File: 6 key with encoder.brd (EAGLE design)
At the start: 96.4 x 40.5 mm, 25 parts, among them SW1 KEYSWITCH-PLAIN-MXHS-1U, SW2 KEYSWITCH-PLAIN-MXHS-1U, SW3 KEYSWITCH-PLAIN-MXHS-1U, SW4 KEYSWITCH-PLAIN-MXHS-1U, SW5 KEYSWITCH-PLAIN-MXHS-1U, SW6 KEYSWITCH-PLAIN-MXHS-1U

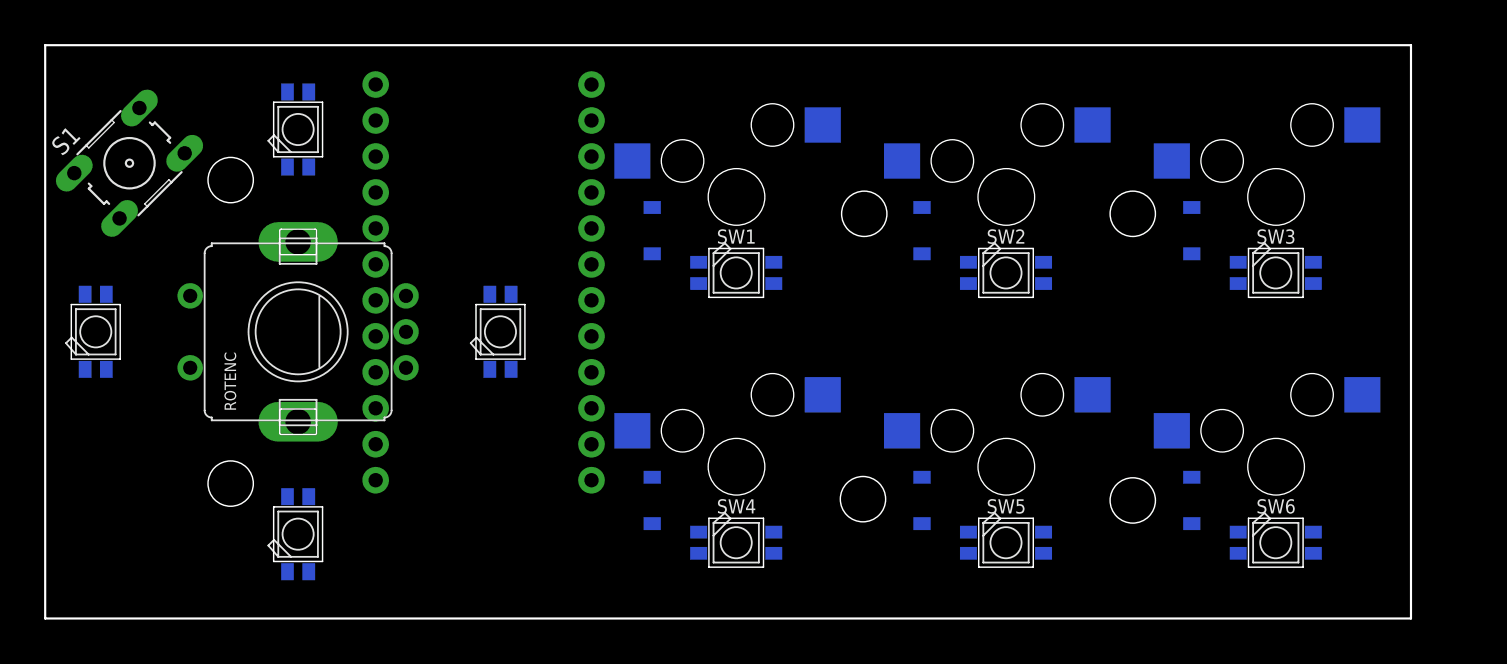
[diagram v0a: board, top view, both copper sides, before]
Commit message: production 12-6-2021
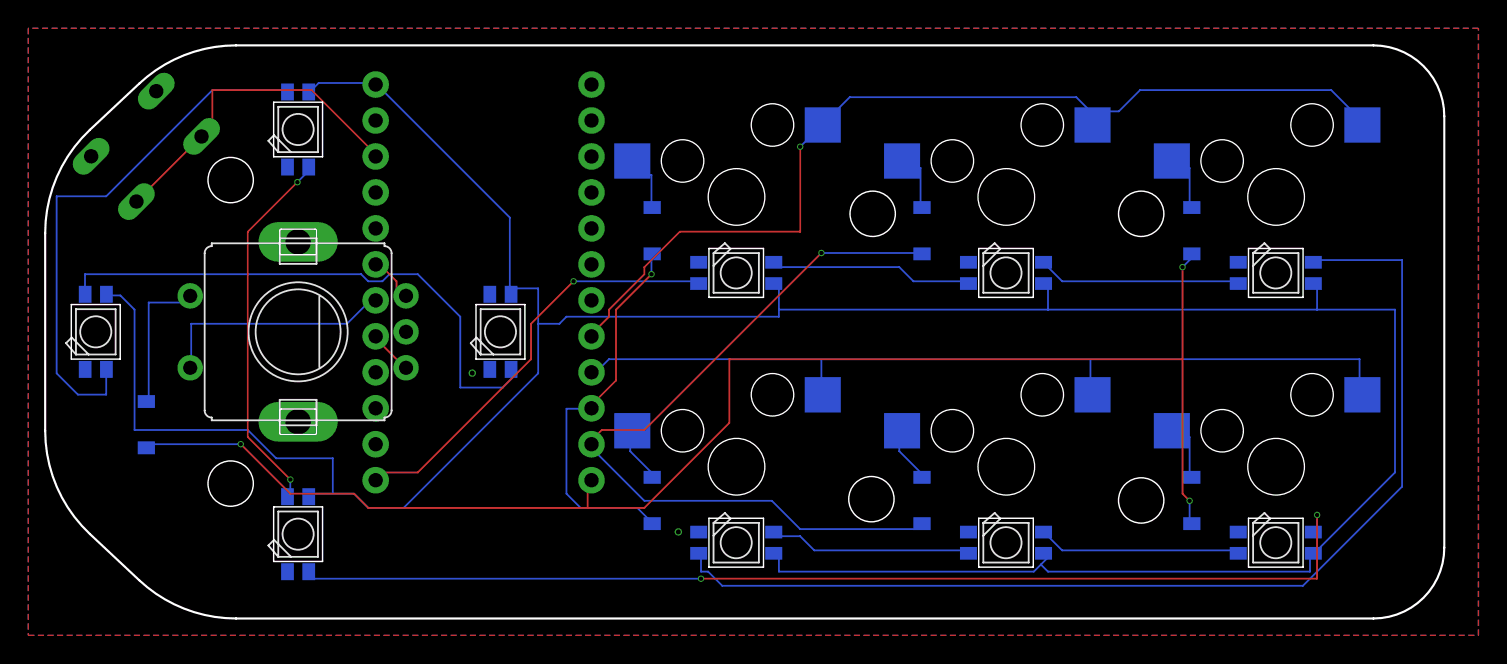
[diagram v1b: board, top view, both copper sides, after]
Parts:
- added D7: (no value), keeb-library:SOD-123
- moved S1 1.68 mm to (8.33, 34.5), flipped to the bottom, turned to 135 degrees
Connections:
- removed net N$24: ROTENC.P$A
- removed net N$25: ROTENC.P$B
- removed net N$26: ROTENC.P$1
- new net ENC_A: B1.17, ROTENC.P$A
- new net ENC_B: B1.19, ROTENC.P$B
- new net N$7: D7.A, ROTENC.P$2
- new net ROW2: B1.18, ROTENC.P$1
- net COL2: now also D7.C
- net GND: no longer ROTENC.P$2
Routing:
- net 5.0V: track 0.00 -> 209.5 mm
- net COL2: track 0.00 -> 103.8 mm, vias 0 -> 3
- net N$15: track 0.00 -> 77.4 mm, vias 0 -> 2
- net N$12: track 0.00 -> 76.5 mm
- net ROW0: track 0.00 -> 70.0 mm, vias 0 -> 1
- net ROW1: track 0.00 -> 62.6 mm
- net COL1: track 0.00 -> 55.5 mm, vias 0 -> 1
- net N$18: track 0.00 -> 39.5 mm
- net N$17: track 0.00 -> 37.8 mm
- net LED: track 0.00 -> 30.4 mm, vias 0 -> 1
- net COL0: track 0.00 -> 27.3 mm, vias 0 -> 1
- net N$16: track 0.00 -> 26.6 mm, vias 0 -> 2
- net RESET: track 0.00 -> 23.6 mm
- net ROW2: track 0.00 -> 16.9 mm
- net N$11: track 0.00 -> 14.3 mm
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- added copper zone on layer 1, net GND
- added copper zone on layer 16, net GND
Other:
- board size 96.4 x 40.5 mm -> 98.8 x 40.5 mm
- board text added: "FUNKFINGER E+6"
- board text added: "https://j.wigg.in/E6 2021.12.02"
